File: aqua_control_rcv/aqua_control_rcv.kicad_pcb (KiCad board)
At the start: 2 copper layers, 88.2 x 68 mm, 51 parts, among them J1 USB_C, J4 Conn_01x03, J5 Conn_01x03, Q1 MMBT2222A, Q2 IRLML6402, SW1 RESET, SW2 BOOT, SW3 BOOT, SW4 BOOT, U1 ESP32-S3-WROOM-1, U2 LM1117-3.3, U3 RA-02_LORA

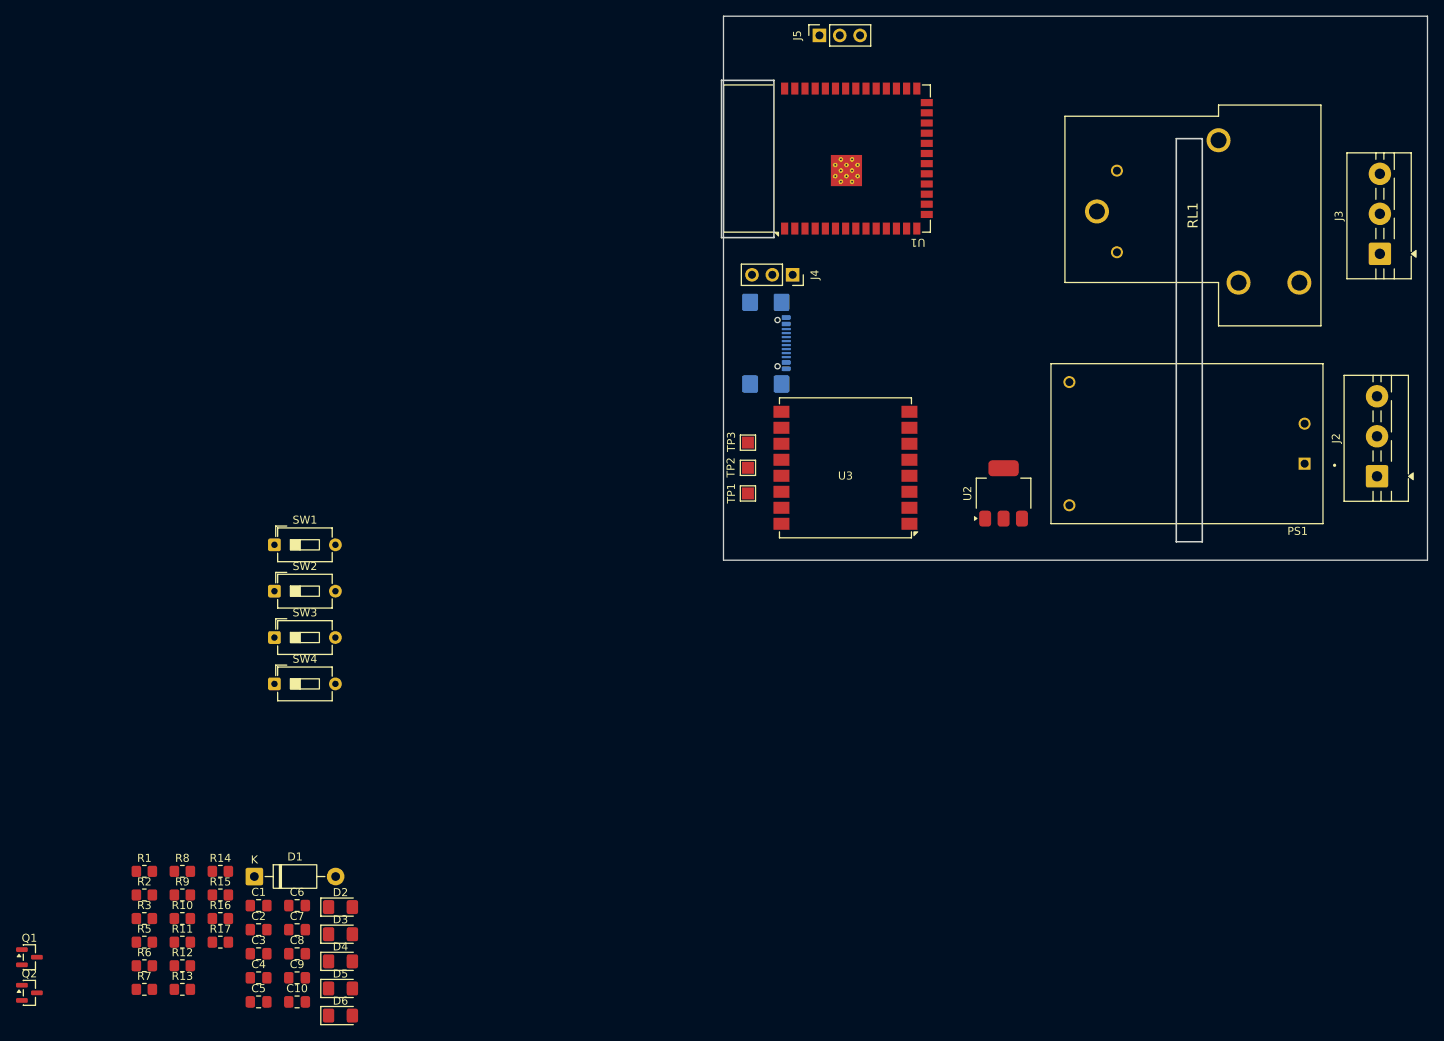
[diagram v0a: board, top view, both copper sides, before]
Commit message: routing completed
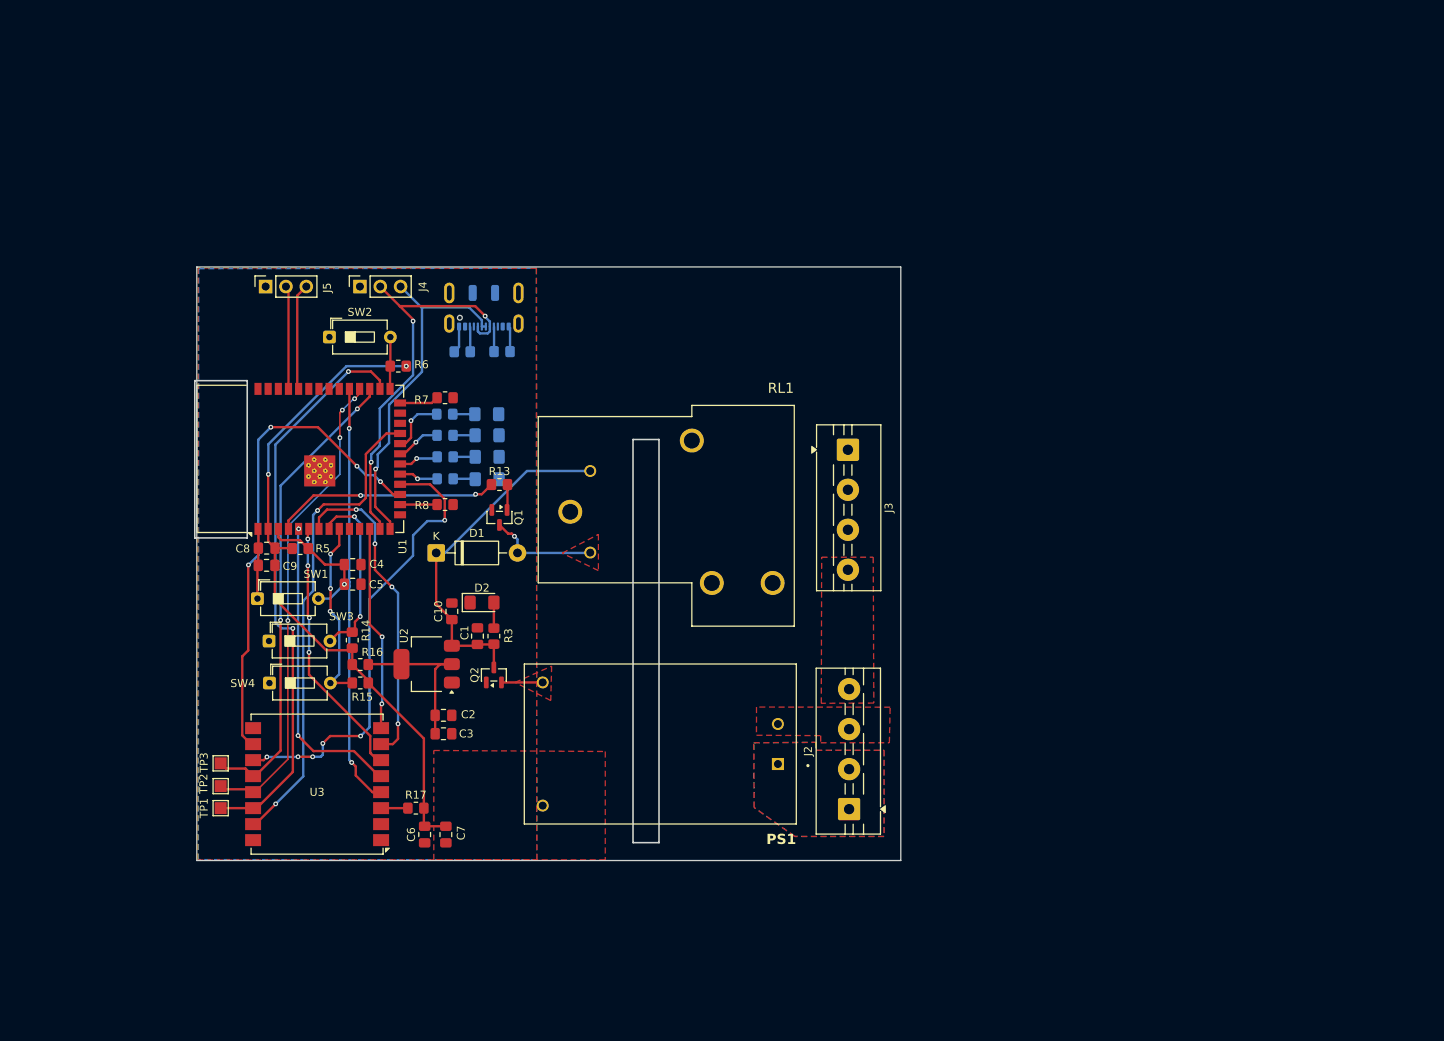
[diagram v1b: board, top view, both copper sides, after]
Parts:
- D3, D4, D5, D6, R1, R10, R11, R12, R2, R9: moved to B.Cu
- J1: footprint Connector_USB:USB_C_Receptacle_GCT_USB4110 -> Connector_USB:USB_C_Receptacle_JAE_DX07S016JA1R1500
- J2, J3: value ~ -> Screw_Terminal_01x04; footprint TerminalBlock:TerminalBlock_MaiXu_MX126-5.0-03P_1x03_P5.00mm -> TerminalBlock:TerminalBlock_MaiXu_MX126-5.0-04P_1x04_P5.00mm
- moved R7 83.0 mm to (147.6, 67.5), turned to 180 degrees
- moved R6 81.4 mm to (141.8, 63.5)
- moved R2 81.3 mm to (154.7, 61.7), turned to 180 degrees
- moved Q1 80.5 mm to (154.4, 82.5), turned to -90 degrees
- moved J2 78.0 mm to (198.1, 118.9)
- moved D6 77.4 mm to (152.8, 69.5), turned to 180 degrees
- moved TP3 77.1 mm to (119.6, 113.2)
- moved TP2 77.0 mm to (119.6, 116.0)
- moved U3 77.0 mm to (131.6, 115.8)
- moved TP1 76.8 mm to (119.6, 118.8)
- moved R12 76.3 mm to (147.6, 69.5)
- moved R1 76.1 mm to (149.8, 61.7), turned to 180 degrees
- moved J5 76.0 mm to (125.2, 53.6)
- moved PS1 75.8 mm to (174.5, 110.8)
- moved RL1 75.8 mm to (163.3, 81.7)
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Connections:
- J2 pad 2: N_in -> L_in
- J2 pad 3: Earth -> N_in
- J3 pad 2: N_in -> L_out
- J3 pad 3: Earth -> N_in
- R16 pad 1: 3.3v -> Net-(U2-VO)
- R16 pad 2: Net-(U2-VO) -> 3.3v
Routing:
- net 3.3v: track 0.00 -> 84.3 mm, vias 0 -> 2
- net MOSI: track 0.00 -> 71.9 mm, vias 0 -> 2
- net DIO4: track 0.00 -> 61.4 mm, vias 0 -> 4
- net MISO: track 0.00 -> 60.5 mm, vias 0 -> 4
- net NSS: track 0.00 -> 60.2 mm, vias 0 -> 2
- net SCK: track 0.00 -> 59.3 mm, vias 0 -> 2
- net DIO5: track 0.00 -> 56.9 mm, vias 0 -> 6
- net RST: track 0.00 -> 52.7 mm, vias 0 -> 2
- net D-: track 0.00 -> 50.2 mm, vias 0 -> 3
- net 5v: track 0.00 -> 44.2 mm
- net D+: track 0.00 -> 44.1 mm, vias 0 -> 1
- net DIO2: track 0.00 -> 40.2 mm, vias 0 -> 4
- net DIO0: track 0.00 -> 38.4 mm, vias 0 -> 2
- net DIO1: track 0.00 -> 33.1 mm, vias 0 -> 4
- net RELAY: track 0.00 -> 28.3 mm, vias 0 -> 2
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- added copper zone on F.Cu, net C
- added copper zone on F.Cu, net Earth
- added copper zone on B.Cu, net GND
- added copper zone on F.Cu, net GND
- added copper zone on B.Cu, net L_in
- added copper zone on F.Cu, net L_in
- added copper zone on F.Cu, net N_in
- added copper zone on F.Cu, net Vin
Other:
- board size 88.2 x 68 mm -> 88.2 x 74.2 mm
